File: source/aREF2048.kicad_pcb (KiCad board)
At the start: 2 copper layers, 63.2 x 21 mm, 34 parts, among them J1 BATT, J2 VREF, J3 GND, Q1 IRLML6401, U1 TPS3809K33, U2 LTC6655CHMS8-2.048, U3 LTC2054, U4 OPA365

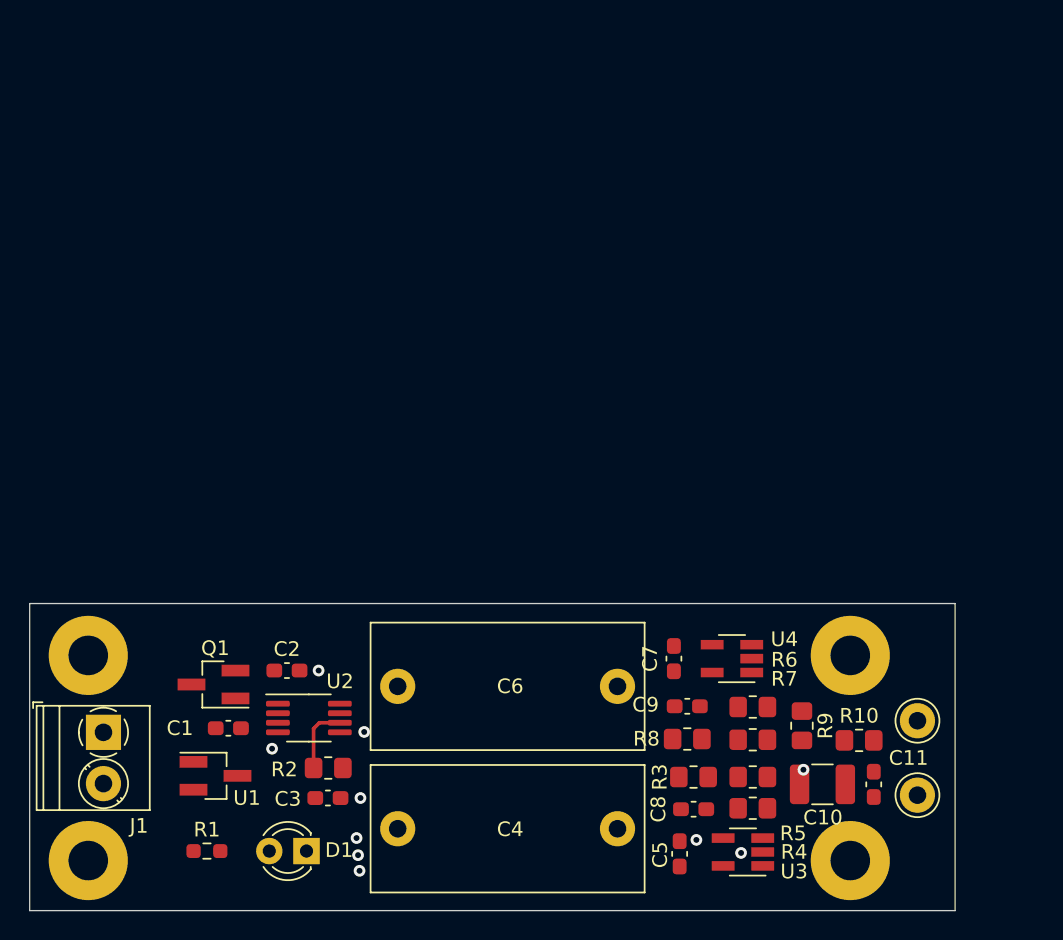
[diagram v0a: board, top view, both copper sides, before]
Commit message: Version 0.1
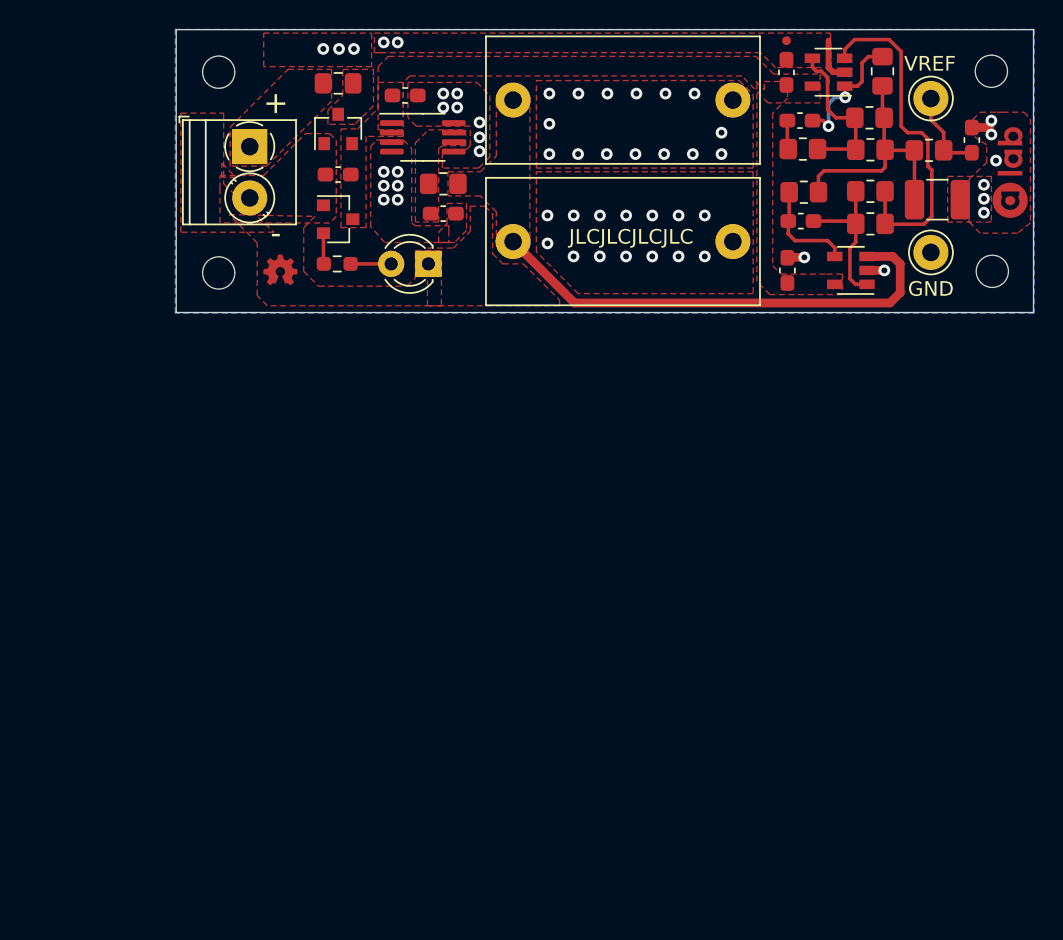
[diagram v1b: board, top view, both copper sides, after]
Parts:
- added F1: 200mA, Fuse:Fuse_0805_2012Metric_Pad1.15x1.40mm_HandSolder, F.Cu at (142.0, 89.0)
- added G***: LOGO, a.lab-kicad-footprints:logo_alab_Copper, F.Cu at (188.7, 95.2)
- added G***: LOGO, gkl_logos:oshw_small, F.Cu at (138.1, 101.7)
- H1, H2, H3, H4: footprint MountingHole:MountingHole_2.7mm_M2.5_Pad -> MountingHole:MountingHole_2.2mm_M2
- Q1, U1: footprint Package_TO_SOT_SMD:SOT-23_Handsoldering -> Package_TO_SOT_SMD:SOT-23
- U3, U4: footprint Package_TO_SOT_SMD:SOT-23-5_HandSoldering -> Package_TO_SOT_SMD:SOT-23-5
- moved R9 45.0 mm to (179.2, 88.1)
- moved C11 44.5 mm to (185.3, 92.8), turned to 90 degrees
- moved J2 42.5 mm to (182.5, 90.0)
- moved H4 41.4 mm to (186.7, 101.8)
- moved J1 41.2 mm to (136.0, 93.3)
- moved H2 41.1 mm to (133.9, 101.9)
- moved R7 41.1 mm to (178.4, 93.5)
- moved R1 41.0 mm to (142.0, 101.3)
- moved R8 41.0 mm to (173.8, 93.4)
- moved H3 41.0 mm to (186.6, 88.1)
- moved R6 41.0 mm to (178.3, 91.3)
- moved D1 40.9 mm to (148.2, 101.3)
- moved C4 40.8 mm to (154.0, 99.8)
- moved C8 40.8 mm to (173.6, 98.4)
- moved H1 40.8 mm to (133.9, 88.2)
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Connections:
- J1 pad 1: Net-(J1-Pad1) -> Net-(F1-Pad2)
- Q1 pad 3: Net-(J1-Pad1) -> Net-(F1-Pad1)
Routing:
- net Net-(C4-Pad1): track 0.00 -> 32.9 mm
- net Net-(R4-Pad1): track 0.00 -> 23.4 mm
- net Net-(C10-Pad1): track 0.00 -> 17.1 mm
- net Net-(R6-Pad1): track 0.00 -> 11.5 mm
- net Net-(C8-Pad2): track 0.00 -> 10.4 mm
- net Net-(C9-Pad2): track 0.00 -> 8.94 mm, vias 0 -> 2
- net Net-(C8-Pad1): track 0.00 -> 7.03 mm
- net GND: track 0.00 -> 6.66 mm, vias 10 -> 55
- net Net-(C11-Pad1): track 0.00 -> 5.89 mm
- net Net-(C3-Pad1): track 4.65 -> 0.00 mm
- net Net-(D1-Pad2): track 0.00 -> 2.77 mm
- net Net-(R1-Pad2): track 0.00 -> 2.11 mm
- net Net-(C9-Pad1): track 0.00 -> 1.97 mm
- added copper zone on B.Cu, net GND
- added copper zone on F.Cu, net GND
- added copper zone on F.Cu, net Net-(C3-Pad1)
- added copper zone on F.Cu, net Net-(C4-Pad1)
- added copper zone on F.Cu, net Net-(F1-Pad1)
- added copper zone on F.Cu, net Net-(F1-Pad2)
- added copper zone on F.Cu, net VCC
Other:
- board size 63.2 x 21 mm -> 58.5 x 19.3 mm
- board text added: "+"
- board text added: "-"
- board text added: "GND"
- board text added: "JLCJLCJLCJLC"
- board text added: "VREF"
